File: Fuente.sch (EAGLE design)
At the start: 33 parts

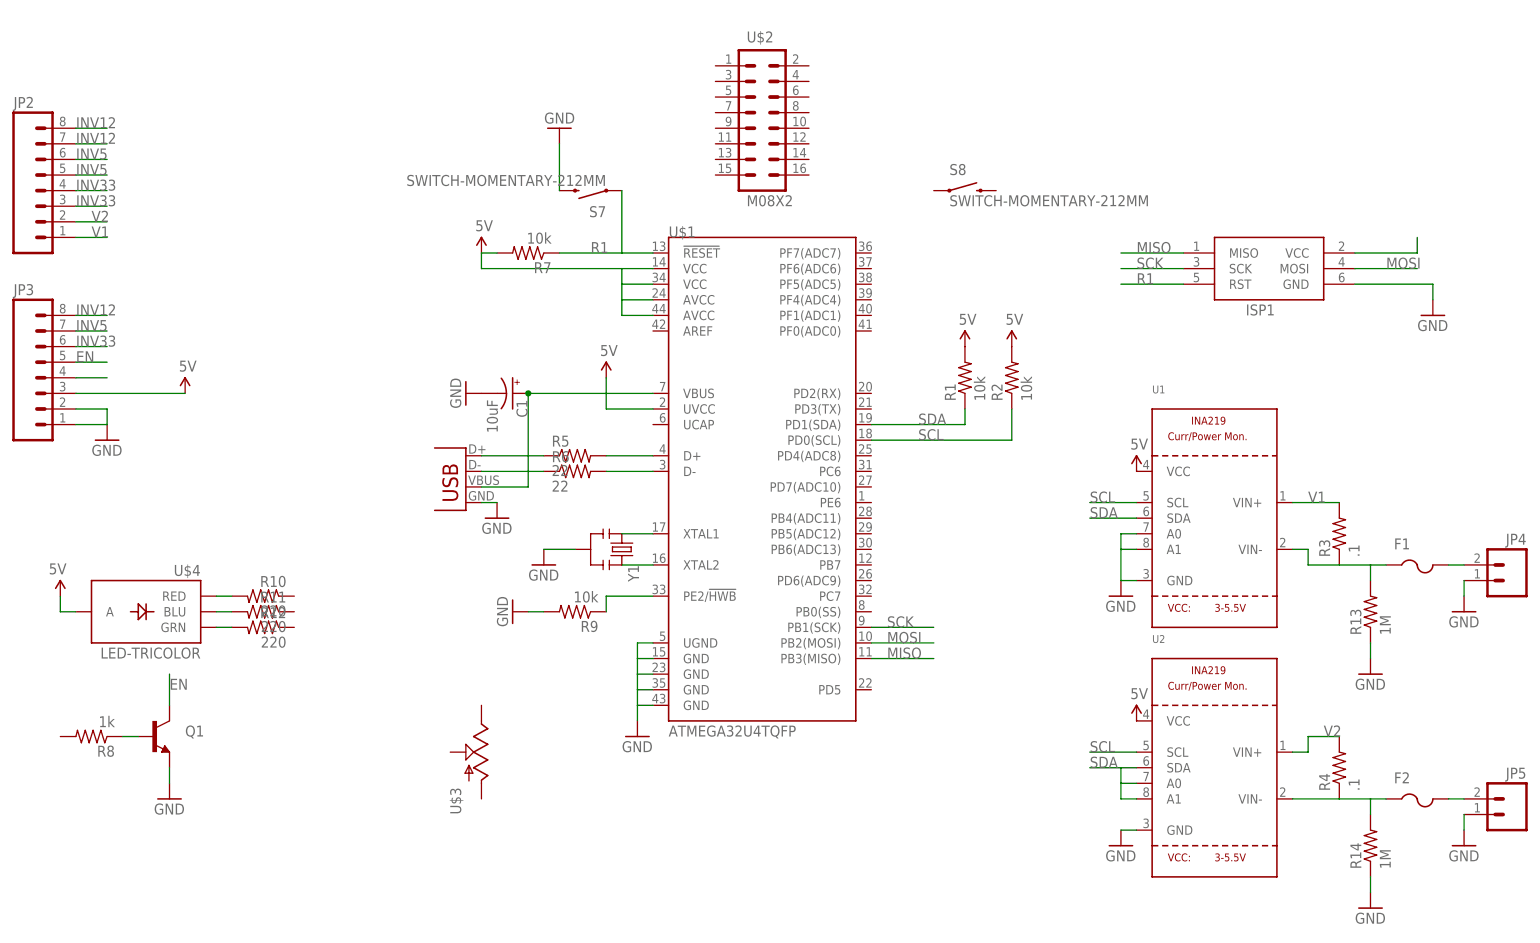
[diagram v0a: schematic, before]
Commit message: pcb and sch updated
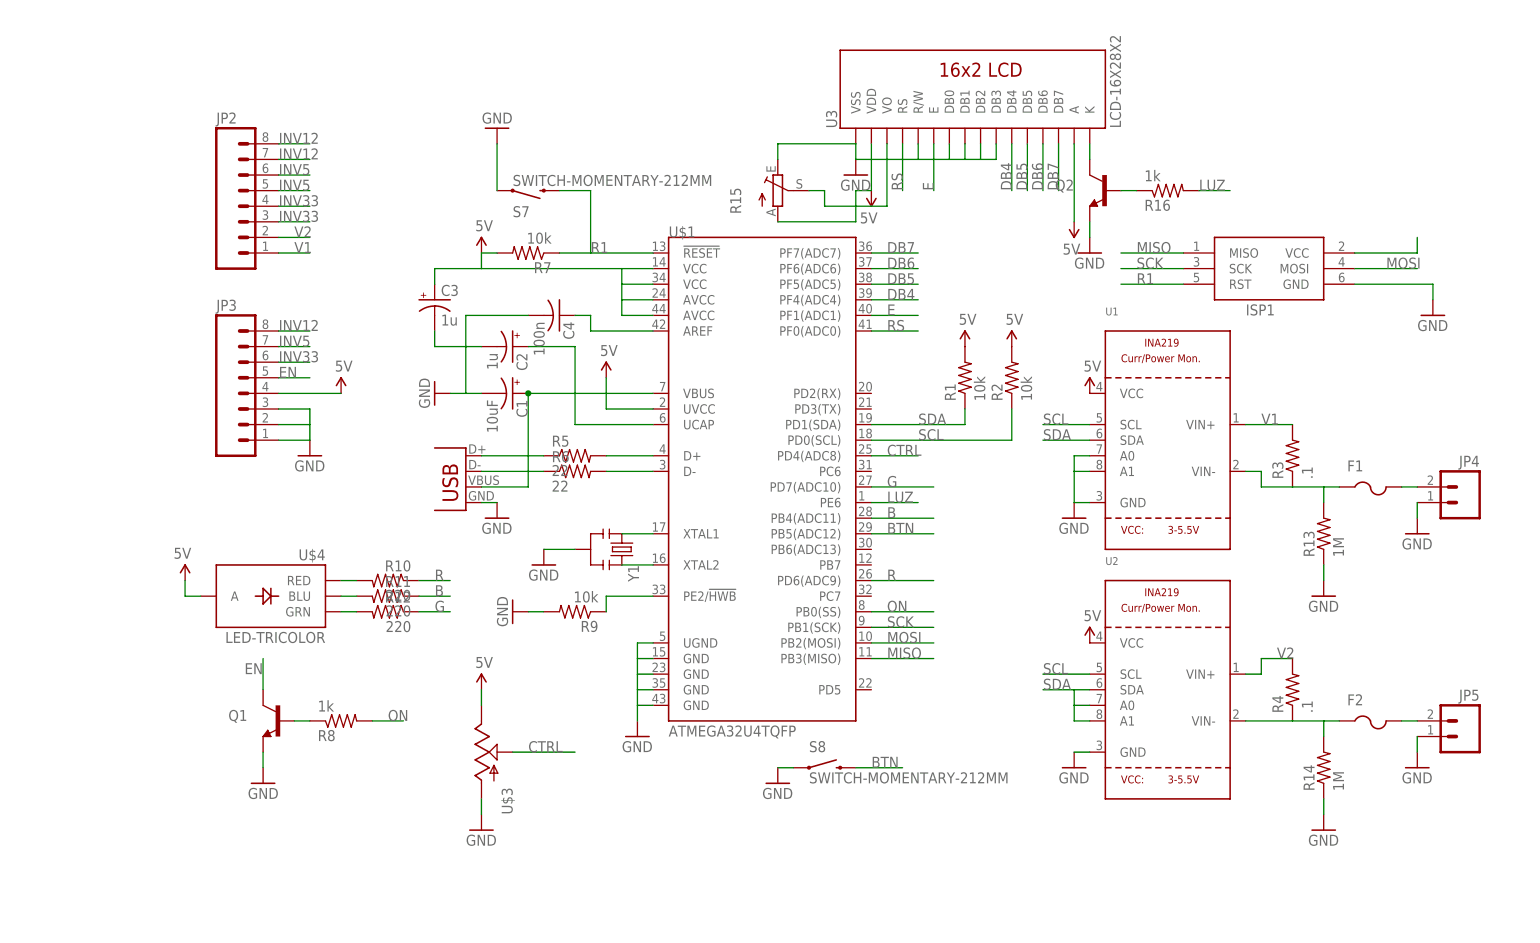
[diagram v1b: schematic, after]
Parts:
- removed U$2: M08X2, SparkFun-Connectors:M08X2
- added C2, C3: 1u, adafruit:CPOL-USE2.5-6
- added C4: 100n, adafruit:C-USC0805K
- added Q2: (no value), SparkFun-DiscreteSemi:TRANSISTOR_NPNSOT23
- added R15: (no value), pot:TRIM_EU-CT6
- added R16: 1k, adafruit:R-US_M0805
- added U3: LCD-16X28X2, SparkFun-Displays:LCD-16X28X2
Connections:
- new net B: R11.1, U$1.PB4(ADC11)
- new net BTN: S8.2, U$1.PB5(ADC12)
- new net CTRL: U$1.PD4(ADC8), U$3.S
- new net DB4: U$1.PF4(ADC4), U3.DB4
- new net DB5: U$1.PF5(ADC5), U3.DB5
- new net DB6: U$1.PF6(ADC6), U3.DB6
- new net DB7: U$1.PF7(ADC7), U3.DB7
- new net E: U$1.PF1(ADC1), U3.E
- new net G: R12.1, U$1.PD7(ADC10)
- new net LUZ: R16.2, U$1.PE6
- new net N$18: C4.1, U$1.AREF
- new net N$21: R15.S, U3.VO
- new net N$22: C2.+, U$1.UCAP
- new net N$29: Q2.C, U3.K
- new net ON: R8.2, U$1.PB0(SS)
- new net R: R10.1, U$1.PD6(ADC9)
- new net RS: U$1.PF0(ADC0), U3.RS
- net 5V: now also C3.+, JP3.4, R15.A, U$3.E, U3.A, U3.VDD; no longer JP3.3
- net GND: now also C2.-, C3.-, C4.2, JP3.3, Q2.E, R15.E, S7.1, S8.1, U$3.A, U3.DB0, U3.DB1, U3.DB2, U3.DB3, U3.R/W, U3.VSS; no longer S7.2
- net N$19: now also Q2.B, R16.1; no longer JP3.4
- net R1: now also S7.2; no longer S7.1
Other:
- moved on the sheet: F1, F2, JP2, JP3, JP4, JP5, Q1, R10, R11, R12, R13, R14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
